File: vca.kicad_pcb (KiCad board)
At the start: 2 copper layers, 59.7 x 128.5 mm, 65 parts, among them J1 Signal 1, J2 Signal 2, J3 CV 1, J4 CV 2, J5 Out 1, J6 Out 2, J7 Conn_02x05_Odd_Even, Q1 BCM847, Q2 BC547C, U1 TL074

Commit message: prepping for initial manu
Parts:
- added TP1: TestPoint, TestPoint:TestPoint_Plated_Hole_D2.0mm, B.Cu at (30.5, 84.1)
- H6: value Control lvl -> control lvl
- moved H1 225.3 mm to (24.1, 129.2)
- moved H2 225.3 mm to (41.9, 129.2)
- moved H3 225.3 mm to (24.1, 251.8)
- moved H4 225.3 mm to (41.9, 251.8)
- moved H10 225.3 mm to (25.4, 215.9)
- moved H11 225.3 mm to (40.6, 215.9)
- moved H12 225.3 mm to (25.4, 238.8)
- moved H13 225.3 mm to (40.6, 238.8)
- moved H14 225.3 mm to (43.2, 157.5)
- moved H5 225.3 mm to (33.0, 167.6)
- moved H6 225.3 mm to (33.0, 193.0)
- moved H7 225.3 mm to (33.0, 142.2)
- moved H8 225.3 mm to (25.4, 227.3)
- moved H9 225.3 mm to (40.6, 227.3)
- moved C4 165.4 mm to (22.9, 28.0)
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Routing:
- net Net-(R10-Pad2): track 6.64 -> 15.2 mm, vias 0 -> 1
- net Net-(R15-Pad1): track 16.8 -> 18.0 mm
- net Net-(J4-PadT): track 24.3 -> 24.9 mm
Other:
- board size 59.7 x 128.5 mm -> 30.5 x 239.5 mm
- board text added: "1 cv 2"
- board text added: "1 in 2"
- board text added: "1 out 2"
- board text added: "control lvl"
- board text added: "gain"
- board text added: "input lvl"

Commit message: sent to manu
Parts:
- moved C2 2.54 mm to (36.2, 86.3)
- moved J1 2.54 mm to (25.4, 108.0)
- moved J2 2.54 mm to (40.6, 108.0)
- moved Q1 2.54 mm to (43.5, 74.9)
- moved R13 2.54 mm to (32.4, 80.0)
- moved R14 2.54 mm to (24.1, 80.0)
- moved R15 2.54 mm to (24.1, 76.2)
- moved R16 2.54 mm to (24.1, 78.1)
- moved R17 2.54 mm to (24.1, 74.3)
- moved R18 2.54 mm to (28.6, 80.0)
- moved R19 2.54 mm to (30.5, 82.8)
- moved R2 2.54 mm to (36.8, 71.1)
- moved R21 2.54 mm to (43.2, 69.2)
- moved R3 2.54 mm to (36.8, 67.3)
- moved R4 2.54 mm to (36.8, 69.2)
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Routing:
- net Net-(J4-PadT): track 24.9 -> 33.9 mm
- net Net-(R15-Pad1): track 18.0 -> 24.7 mm
- net GND: track 125.5 -> 130.4 mm, vias 5 -> 7
- net Net-(R10-Pad2): track 15.2 -> 14.3 mm
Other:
- board size 30.5 x 239.5 mm -> 30 x 237.9 mm

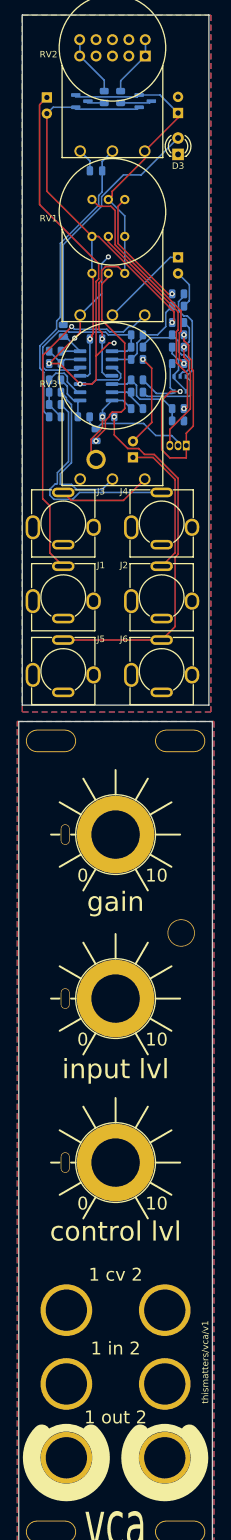
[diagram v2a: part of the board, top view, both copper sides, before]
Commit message: v2 ready
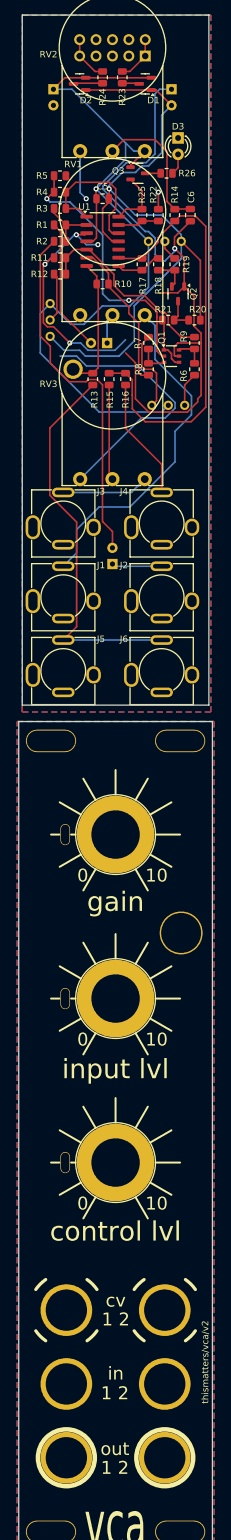
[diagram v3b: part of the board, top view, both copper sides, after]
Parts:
- added Q3: BC847C, Package_TO_SOT_SMD:SOT-23-3, F.Cu at (37.0, 42.3)
- C5, C6, D1, D2, Q1, R1, R10, R11, R12, R13, R14, R15, R16, R17, R18, R19, R2, R20, R21, R23, R24, R3, R4, R5, R6, R7, R8, R9, U1: moved to F.Cu
- H10, H11: footprint eurorack:Mech-AudioJack-Hole -> eurorack:Mech-AudioJack-Hole-Input-CV
- H14: footprint eurorack:Mech-LED-Hole-4mm -> eurorack:Mech-LED-Hole-3mm-Bezel
- H6: value control lvl -> Control lvl
- H8, H9: footprint eurorack:Mech-AudioJack-Hole -> eurorack:Mech-AudioJack-Hole-Input
- Q2: value BC547C -> BC847C; footprint Package_TO_SOT_THT:TO-92L_Inline -> Package_TO_SOT_SMD:SOT-23-3; moved to F.Cu
- R22, R25: value 1K -> 100K; moved to F.Cu
- R26: value 100 -> 1K; moved to F.Cu
- RV1: value 100K LOG* -> A100K
- RV2, RV3: value 100K LOG* -> B100K
- moved R14 36.3 mm to (42.7, 48.8), turned to -90 degrees
- moved RV4 35.0 mm to (44.2, 78.2), turned to 0 degrees
- moved R11 31.2 mm to (24.9, 55.4), turned to 0 degrees
- moved R5 30.7 mm to (24.9, 42.7)
- moved R26 29.2 mm to (41.4, 42.3), turned to 180 degrees
- moved R19 29.1 mm to (42.7, 56.4), turned to -90 degrees
- moved R22 28.0 mm to (40.1, 48.8), turned to 90 degrees
- moved R12 27.7 mm to (24.9, 57.9), turned to 0 degrees
- moved R4 26.8 mm to (24.9, 45.2), turned to 180 degrees
- moved R18 26.3 mm to (40.1, 56.4), turned to -90 degrees
- moved R25 25.0 mm to (37.6, 48.8), turned to 90 degrees
- moved Q2 23.5 mm to (43.2, 61.0), turned to -90 degrees
- moved R3 22.9 mm to (24.9, 47.8), turned to 0 degrees
- moved R17 22.4 mm to (37.6, 56.4), turned to -90 degrees
- moved R1 22.2 mm to (24.9, 50.3), turned to 0 degrees
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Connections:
- R25 pad 2: Net-(R25-Pad2) -> Net-(Q3-B)
- R26 pad 2: Net-(R25-Pad2) -> Net-(Q3-E)
- U1 pad 14: Net-(R25-Pad2) -> Net-(Q3-B)
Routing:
- net GND: track 130.4 -> 191.5 mm
- net +12V: track 69.7 -> 125.7 mm
- net Net-(U1C--): track 13.4 -> 67.0 mm
- net Net-(C2-Pad2): track 14.4 -> 56.0 mm, vias 1 -> 0
- net Net-(D3-A): track 37.9 -> 3.28 mm
- net Net-(R6-Pad2): track 32.6 -> 5.30 mm, vias 1 -> 0
- net Net-(R19-Pad1): track 30.5 -> 3.28 mm, vias 1 -> 0
- net Net-(Q1A-B1): track 14.2 -> 41.2 mm, vias 0 -> 2
- net -12V: track 79.3 -> 105.4 mm, vias 2 -> 1
- net Net-(R12-Pad1): track 32.4 -> 7.71 mm, vias 1 -> 0
- net Net-(C6-Pad1): track 46.4 -> 21.8 mm
- net Net-(Q1B-C2): track 25.6 -> 4.71 mm
- net Net-(U1B--): track 5.89 -> 23.4 mm
- net Net-(Q2-E): track 21.5 -> 5.42 mm, vias 1 -> 0
- net Net-(U1B-+): track 14.3 -> 30.3 mm
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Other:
- board text added: "1 2"
- board text added: "cv"
- board text added: "in"
- board text added: "out"
- board text added: "thismatters/vca/v2"
- board text removed: "1 cv 2"
- board text removed: "1 in 2"
- board text removed: "1 out 2"
- board text removed: "thismatters/vca/v1"

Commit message: correcting some BOM issues
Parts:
- Q2, Q3: value BC847C -> BC547C
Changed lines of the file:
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@@
         (effects (font (size 1 1) (thickness 0.15)))
     )
-    (fp_text value "BC847C" (at 0 2.4) (layer "F.Fab")
+    (fp_text value "BC547C" (at 0 2.4) (layer "F.Fab")
         (effects (font (size 1 1) (thickness 0.15)))
     )
@@
         (effects (font (size 1 1) (thickness 0.15)))
     )
-    (fp_text value "BC847C" (at 0 2.4 90) (layer "F.Fab")
-        (effects (font (size 1 1) (thickness 0.15)))
-    )
+    (fp_text value "BC547C" (at 0 2.4 90) (layer "F.Fab")
+        (effects (font (size 1 1) (thickness 0.15)))
+    )
